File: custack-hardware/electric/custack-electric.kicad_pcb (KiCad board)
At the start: 2 copper layers, 92 x 65 mm, 102 parts, among them J1 XH 2.5mmピッチ 2極 オス AWG22, J10 PH 2mmピッチ 3極 オス AWG24, J11 PH 2mmピッチ 3極 オス AWG24, J12 PH 2mmピッチ 3極 オス AWG24, J13 4P MMale magnetic connector (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, J14 PH 2mmピッチ 3極 オス AWG24, J15 PH 2mmピッチ 2極 オス AWG24, J16 4P MMale magnetic connector (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, J17 PH 2mmピッチ 3極 オス AWG24, J18 PH 2mmピッチ 2極 オス AWG24, J2 XH 2.5mmピッチ 2極 オス AWG24, J3 2x15P@2.54mm SMD, J4 PH 2mmピッチ 4極 オス AWG24, J5 PH 2mmピッチ 4極 オス AWG24, J6 PH 2mmピッチ 4極 オス AWG24, J7 4P MMale magnetic connector (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, J8 PH 2mmピッチ 3極 オス AWG24, J9 PH 2mmピッチ 3極 オス AWG24, Q1 MOSFET P-CH 20V 6A SOT23F, Q2 N-ch 30V 4A SOT23F, Q3 N-ch 30V 4A SOT23F, Q4 N-ch 30V 4A SOT23F, SW1 12V 100mA, U1 IN:4.5V-17V, OUT:0.765V-7V,2A, U10 20MHz 16KB FLASH, U11 Vin(MAX): 13.2V, Vout: 3.3V 2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, U2 20MHz 16KB FLASH, U3 非反転 1.65-5.5V, 32mA SOT-23-5, U4 非反転 1.65-5.5V, 32mA SOT-23-5, U5 Vin(MAX): 13.2V, Vout: 3.3V 2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, U6 非反転 1.65-5.5V, 32mA SOT-23-5, U7 非反転 1.65-5.5V, 32mA SOT-23-5, U8 20MHz 16KB FLASH, U9 Vin(MAX): 13.2V, Vout: 3.3V 2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

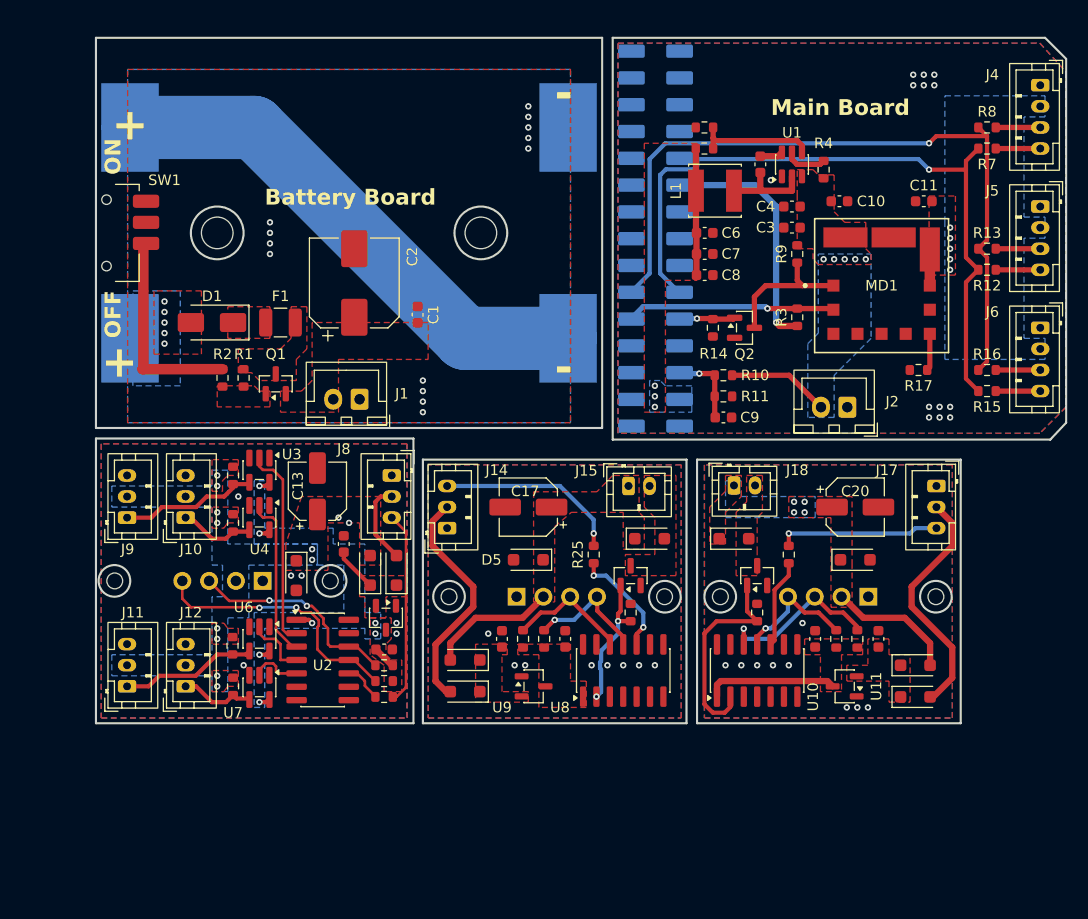
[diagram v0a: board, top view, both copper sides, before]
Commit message: pcb board complete
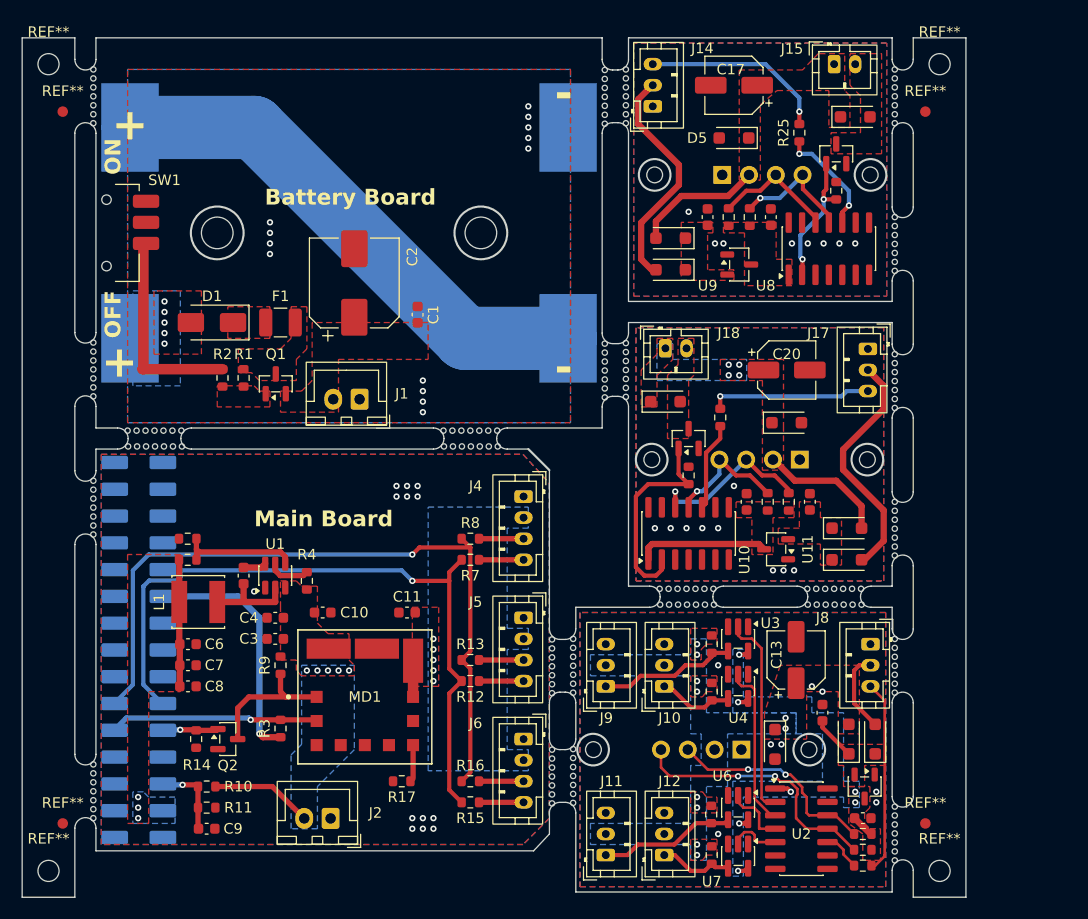
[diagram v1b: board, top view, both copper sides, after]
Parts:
- added REF**: MouseBite-Slot_2.0x4.5mm_outset_D0.5mm_P0.85mm_7h, Panelization:MouseBite-Slot_2.0x4.5mm_outset_D0.5mm_P0.85mm_7h, F.Cu at (82.0, 81.5)
- added REF**: MountingHole_2.1mm, MountingHole:MountingHole_2.1mm, F.Cu at (21.5, 108.5)
- added REF**: MouseBite-Slot_2.0x4.5mm_outset_D0.5mm_P0.85mm_7h, Panelization:MouseBite-Slot_2.0x4.5mm_outset_D0.5mm_P0.85mm_7h, F.Cu at (26.0, 74.0)
- added REF**: MouseBite-Slot_2.0x4.5mm_outset_D0.5mm_P0.85mm_7h, Panelization:MouseBite-Slot_2.0x4.5mm_outset_D0.5mm_P0.85mm_7h, F.Cu at (31.6, 66.5)
- added REF**: Fiducial_1mm_Mask2mm, Fiducial:Fiducial_1mm_Mask2mm, F.Cu at (22.9, 104.0)
- added REF**: MouseBite-Slot_2.0x4.5mm_outset_D0.5mm_P0.85mm_7h, Panelization:MouseBite-Slot_2.0x4.5mm_outset_D0.5mm_P0.85mm_7h, F.Cu at (96.0, 81.5)
- added REF**: MouseBite-Slot_2.0x4.5mm_outset_D0.5mm_P0.85mm_7h, Panelization:MouseBite-Slot_2.0x4.5mm_outset_D0.5mm_P0.85mm_7h, F.Cu at (26.0, 61.0)
- added REF**: Fiducial_1mm_Mask2mm, Fiducial:Fiducial_1mm_Mask2mm, F.Cu at (104.7, 104.0)
- added REF**: MouseBite-Slot_2.0x4.5mm_outset_D0.5mm_P0.85mm_7h, Panelization:MouseBite-Slot_2.0x4.5mm_outset_D0.5mm_P0.85mm_7h, F.Cu at (101.5, 35.0)
- added REF**: MouseBite-Slot_2.0x4.5mm_outset_D0.5mm_P0.85mm_7h, Panelization:MouseBite-Slot_2.0x4.5mm_outset_D0.5mm_P0.85mm_7h, F.Cu at (71.5, 89.0)
- added REF**: MouseBite-Slot_2.0x4.5mm_outset_D0.5mm_P0.85mm_7h, Panelization:MouseBite-Slot_2.0x4.5mm_outset_D0.5mm_P0.85mm_7h, F.Cu at (76.5, 35.0)
- added REF**: MouseBite-Slot_2.0x4.5mm_outset_D0.5mm_P0.85mm_7h, Panelization:MouseBite-Slot_2.0x4.5mm_outset_D0.5mm_P0.85mm_7h, F.Cu at (101.5, 62.0)
- added REF**: MouseBite-Slot_2.0x4.5mm_outset_D0.5mm_P0.85mm_7h, Panelization:MouseBite-Slot_2.0x4.5mm_outset_D0.5mm_P0.85mm_7h, F.Cu at (26.0, 35.0)
- added REF**: MouseBite-Slot_2.0x4.5mm_outset_D0.5mm_P0.85mm_7h, Panelization:MouseBite-Slot_2.0x4.5mm_outset_D0.5mm_P0.85mm_7h, F.Cu at (101.5, 105.0)
- added REF**: MountingHole_2.1mm, MountingHole:MountingHole_2.1mm, F.Cu at (106.0, 108.5)
- added REF**: MouseBite-Slot_2.0x4.5mm_outset_D0.5mm_P0.85mm_7h, Panelization:MouseBite-Slot_2.0x4.5mm_outset_D0.5mm_P0.85mm_7h, F.Cu at (71.5, 99.5)
- added REF**: Fiducial_1mm_Mask2mm, Fiducial:Fiducial_1mm_Mask2mm, F.Cu at (104.7, 36.5)
- added REF**: MountingHole_2.1mm, MountingHole:MountingHole_2.1mm, F.Cu at (106.0, 32.0)
- added REF**: MountingHole_2.1mm, MountingHole:MountingHole_2.1mm, F.Cu at (21.5, 32.0)
- added REF**: MouseBite-Slot_2.0x4.5mm_outset_D0.5mm_P0.85mm_7h, Panelization:MouseBite-Slot_2.0x4.5mm_outset_D0.5mm_P0.85mm_7h, F.Cu at (101.5, 49.0)
- added REF**: MouseBite-Slot_2.0x4.5mm_outset_D0.5mm_P0.85mm_7h, Panelization:MouseBite-Slot_2.0x4.5mm_outset_D0.5mm_P0.85mm_7h, F.Cu at (101.5, 89.0)
- added REF**: MouseBite-Slot_2.0x4.5mm_outset_D0.5mm_P0.85mm_7h, Panelization:MouseBite-Slot_2.0x4.5mm_outset_D0.5mm_P0.85mm_7h, F.Cu at (76.5, 61.0)
- added REF**: MouseBite-Slot_2.0x4.5mm_outset_D0.5mm_P0.85mm_7h, Panelization:MouseBite-Slot_2.0x4.5mm_outset_D0.5mm_P0.85mm_7h, F.Cu at (61.5, 66.5)
- added REF**: Fiducial_1mm_Mask2mm, Fiducial:Fiducial_1mm_Mask2mm, F.Cu at (22.9, 36.5)
- added REF**: MouseBite-Slot_2.0x4.5mm_outset_D0.5mm_P0.85mm_7h, Panelization:MouseBite-Slot_2.0x4.5mm_outset_D0.5mm_P0.85mm_7h, F.Cu at (101.5, 76.0)
- added REF**: MouseBite-Slot_2.0x4.5mm_outset_D0.5mm_P0.85mm_7h, Panelization:MouseBite-Slot_2.0x4.5mm_outset_D0.5mm_P0.85mm_7h, F.Cu at (26.0, 101.0)
- moved C10 62.6 mm to (47.5, 84.0)
- moved C11 62.6 mm to (55.5, 84.0)
- moved C3 62.6 mm to (43.0, 86.5)
- moved C4 62.6 mm to (43.0, 84.5)
- moved C5 62.6 mm to (40.0, 80.5)
- moved C9 62.6 mm to (36.5, 104.5)
- moved J2 62.6 mm to (48.2, 103.5)
- moved J3 62.6 mm to (30.1, 69.8)
- moved J4 62.6 mm to (66.5, 73.0)
- moved J5 62.6 mm to (66.5, 84.5)
- moved J6 62.6 mm to (66.5, 96.0)
- moved L1 62.6 mm to (35.7, 83.0)
- moved MD1 62.6 mm to (51.5, 92.0)
- moved Q2 62.6 mm to (38.5, 96.0)
- moved R10 62.6 mm to (36.5, 100.5)
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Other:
- board size 92 x 65 mm -> 89.5 x 81.5 mm
